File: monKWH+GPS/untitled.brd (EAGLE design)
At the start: 91 x 91 mm, 61 parts, among them J1 U.FL-R-SMT(01), J3 2172034-1, J4 POWER_JACKSLT, Q1 MMBT3904, Q2 MMBT3904, Q3 12MHz, Q4 MC-306, U2 DS1307Z+, U3 MAX3444EASA, U4 AMS1117, U5 MAX232CSE, X1 MSTBA2

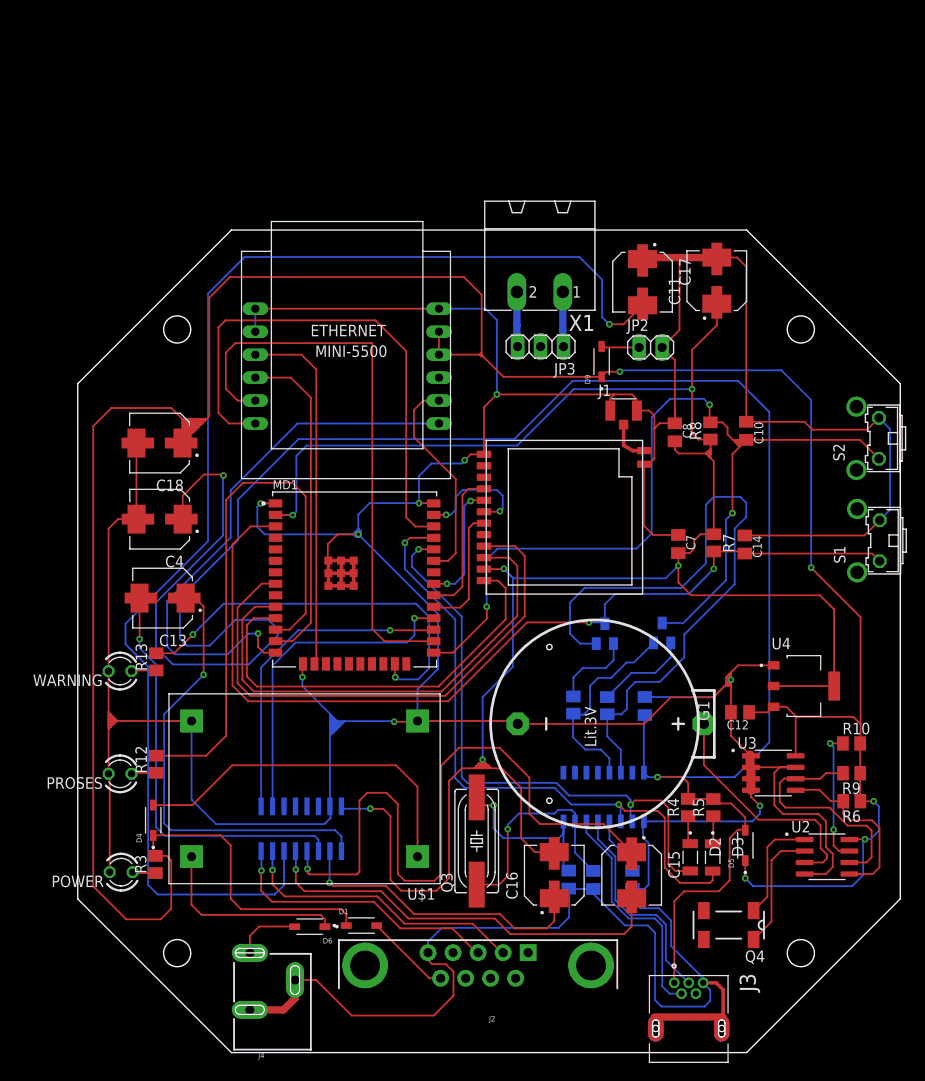
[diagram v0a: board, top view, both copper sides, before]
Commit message: revisi rangkaian
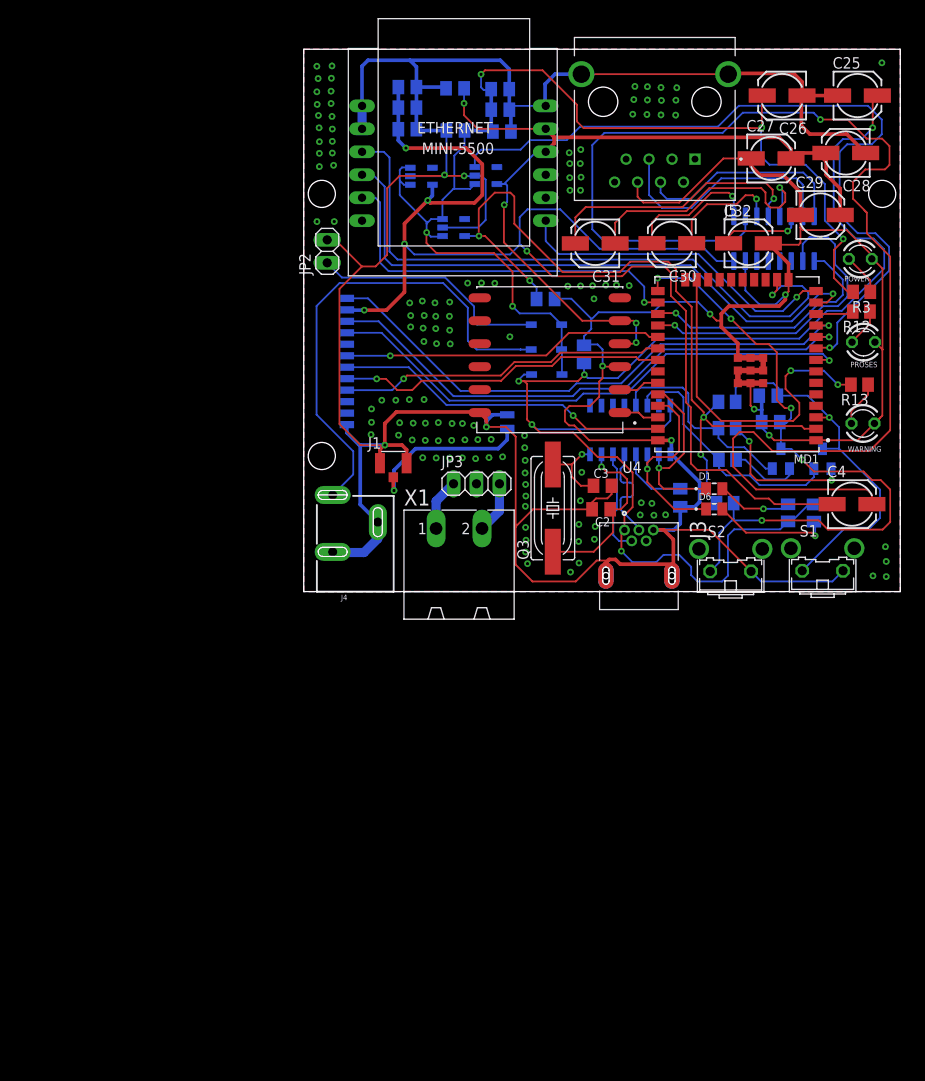
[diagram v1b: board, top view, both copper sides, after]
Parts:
- removed C13, C15, C16, C17, C18: 10uf/50V, EEEFK1H100V:CAP_EEEFK1H100V
- removed D2: Tx, LHN974_RED_LED_1206:LEDC3216X120N
- removed D3: Rx, LHN974_RED_LED_1206:LEDC3216X120N
- removed G1: CR2032H, battery_cr2032:CR2032H
- removed J2: (no value), SparkFun-Connectors:DB9
- removed Q4: MC-306, crystal:MC-306
- removed R10, R6, R9: 10K, adafruit:M0805
- removed U$1: STEPDOWN_SY8205, STEPDOWN_SY8205:STEPDOWN_SY8205
- added C19, C20, C21, C5, C9: 10uF, rcl:C0805K
- added C25: 10uF/16v, rcl:153CLV-0505
- added C26, C28, C30, C31, C32: 10uF/16V, rcl:153CLV-0505
- added C27: 0.1uF/16V, rcl:153CLV-0505
- added C29: 0.1uf/16V, rcl:153CLV-0505
- added J5: RJ45-8N-B, RJ45-8N-B:TE_RJ45-8N-B
- added U1: RT9193-33GB, RT9193-33GB:SOT94P279X129-5N
- C11: value 10uf/50V -> 10uF; device EEEFK1H100V:CAP_EEEFK1H100V -> rcl:C0805K
- C4: value 10uf/50V -> 10uF/16V; device EEEFK1H100V:CAP_EEEFK1H100V -> rcl:153CLV-0505
- D1, D6: value 1N5819HW-7 -> SML-LXT0805IW-TR; device 1N5819HW-7:SOD3715X145N -> SML-LXT0805IW-TR:LEDC2012X120N
- U2: value DS1307Z+ -> RT9193-33GB; device DS1307Z_:SOIC127P600X175-8N -> RT9193-33GB:SOT94P279X129-5N
- U3: value MAX3444EASA -> RT9193-33GB; device MAX3444EASA:SOIC127P600X175-8N -> RT9193-33GB:SOT94P279X129-5N
- U4: value AMS1117 -> L80-R; device AMS1117:SOT229P700X180-4N -> L80-R:XCVR_L80-R
- moved POWER 106.3 mm to (75.6, 76.8), turned to 0 degrees
- moved R3 100.6 mm to (75.7, 73.2), turned to 180 degrees
- moved PROSES 95.1 mm to (75.9, 67.6), turned to 0 degrees
- moved R12 92.7 mm to (75.7, 71.0), turned to 180 degrees
- moved U2 87.7 mm to (27.0, 86.0), flipped to the bottom, turned to 180 degrees
- moved WARNING 86.6 mm to (75.9, 58.6), turned to 0 degrees
- moved U5 83.6 mm to (66.0, 79.0), turned to 270 degrees
- moved R13 83.6 mm to (75.5, 62.9), turned to 180 degrees
- moved C4 76.6 mm to (74.7, 49.7), turned to 0 degrees
- moved U3 73.4 mm to (34.2, 86.0), flipped to the bottom, turned to 180 degrees
- moved C12 71.7 mm to (30.8, 91.0), flipped to the bottom, turned to 0 degrees
- moved D4 67.9 mm to (40.8, 66.8), flipped to the bottom, turned to 0 degrees
- moved D6 64.3 mm to (59.4, 49.1), turned to 0 degrees
- moved D1 62.1 mm to (59.4, 51.4)
- moved D5 56.5 mm to (40.9, 64.0), flipped to the bottom, turned to 0 degrees
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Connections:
- removed net CLK: MD1.20
- removed net CMD: MD1.19
- removed net IO34: MD1.6
- removed net IO35: MD1.7
- removed net N$11: D4.A, U$1.OUT_VCC
- removed net N$15: G1.+, U2.3
- removed net N$18: R10.1, U2.7
- removed net N$20: D1.A, J2.9
- removed net N$23: D6.A, J4.PWR
- removed net N$7: Q4.4, U2.2
- removed net NC: MD1.32
- removed net RST_LAN: MD1.33, U$3.RST
- removed net SCL: R9.2, U2.6, U3.6
- removed net SD0: MD1.21
- removed net SD1: MD1.22
- removed net SD2: MD1.17
- removed net SD3: MD1.18
- removed net SDA: R6.2, U2.5, U3.5
- removed net SENSOR_VN: MD1.5
- removed net SENSOR_VP: MD1.4
- removed net VCC_DB9: D6.C, U$1.IN_VCC
- new net 3V3-LAN-GPS: C21.1, C27.+, C28.+, C29.+, U$3.3V3, U$3.3V3.2, U3.5, U4.4, U4.5
- new net 3V3-LORA-RS232: C19.1, C4.-, C7.2, C8.2, LORA-NICERF-V1.VCC, U2.5, U5.16
- new net EN-3V3-LAN-GPS: MD1.9, U3.3
- new net GPS_RXD: MD1.36, U4.1
- new net GPS_TXD: MD1.33, U4.2
- net 3V3: now also C9.1, U1.5; no longer C11.1, C16.2, C7.2, C8.2, LORA-NICERF-V1.VCC, U4.2, U4.4, U5.16
- net GND: now also C19.2, C20.2, C21.2, C25.-, C26.-, C27.-, C28.-, C29.-, C32.+, C5.2, C9.2, J5.10, J5.6, J5.9, U1.2, U2.2, U4.12, U4.3; no longer C17.1, C18.2, C4.2, G1.-, J2.5, U$1.IN_GND, U$1.OUT_GND, U2.4, U3.1, U3.3, U3.4, U3.7, U4.1
- net INT_LAN: no longer MD1.36
- net N$10: now also C30.+; no longer C13.1
- net N$14: now also C30.-; no longer C13.2
- net N$19: now also C31.+; no longer C15.1
- net N$24: now also C31.-; no longer C15.2
- net N$26: now also C4.+; no longer C16.1
- net N$27: now also C32.-; no longer C17.2
- net N$6: now also D4.A, J4.PWR; no longer Q4.1, U2.1
- net N$8: now also D1.A; no longer D2.+
- net N$9: now also D6.A; no longer D3.+
- net OUT+: now also C11.1, C20.1, C26.+, C5.1, U1.1, U1.3, U2.1, U2.3, U3.1; no longer C18.1, D1.C, R10.2, R6.1, R9.1, U$3.3V3, U$3.3V3.2, U2.8, U3.8, U4.3
- net R2IN: now also J5.4; no longer J2.3
- net RX: now also D6.C; no longer D3.-
- net T2OUT: now also J5.5; no longer J2.2
- net TX: now also D1.C; no longer D2.-
- net VCC: now also C25.+; no longer C4.1
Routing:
- net OUT+: track 332.3 -> 131.0 mm
- net 3V3: track 239.6 -> 87.0 mm, vias 6 -> 4
- net GND: track 644.1 -> 491.8 mm, vias 9 -> 134
- net 3V3-LORA-RS232: track 0.00 -> 148.3 mm, vias 0 -> 5
- net N$27: track 146.1 -> 9.35 mm
- net N$26: track 33.3 -> 141.1 mm
- net 3V3-LAN-GPS: track 0.00 -> 92.7 mm, vias 0 -> 4
- net VCC: track 238.6 -> 150.7 mm, vias 2 -> 5
- net EN-3V3-LAN-GPS: track 0.00 -> 85.8 mm, vias 0 -> 1
- net EN: track 103.3 -> 42.1 mm, vias 2 -> 1
- net INT_LAN: track 58.4 -> 0.00 mm
- net LED_PROSES: track 62.0 -> 4.18 mm
- net RX: track 71.4 -> 22.2 mm, vias 2 -> 1
- net RTS: track 74.6 -> 27.5 mm
- net N$19: track 75.5 -> 29.8 mm
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- added copper zone on layer 1, net GND
- added copper zone on layer 16, net GND
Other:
- board size 91 x 91 mm -> 66 x 60 mm
